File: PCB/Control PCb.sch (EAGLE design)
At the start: 7 parts

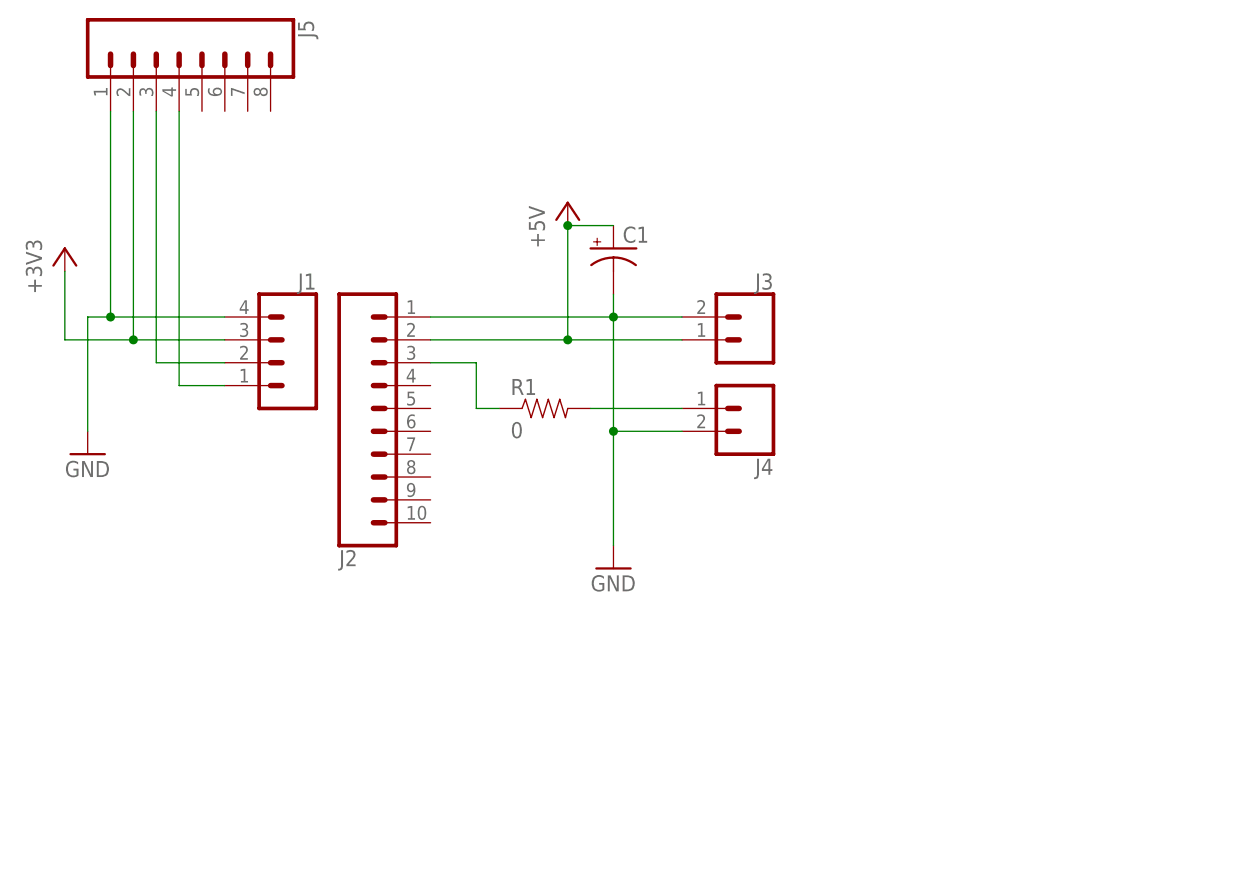
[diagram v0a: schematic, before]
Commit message: PCB files etc
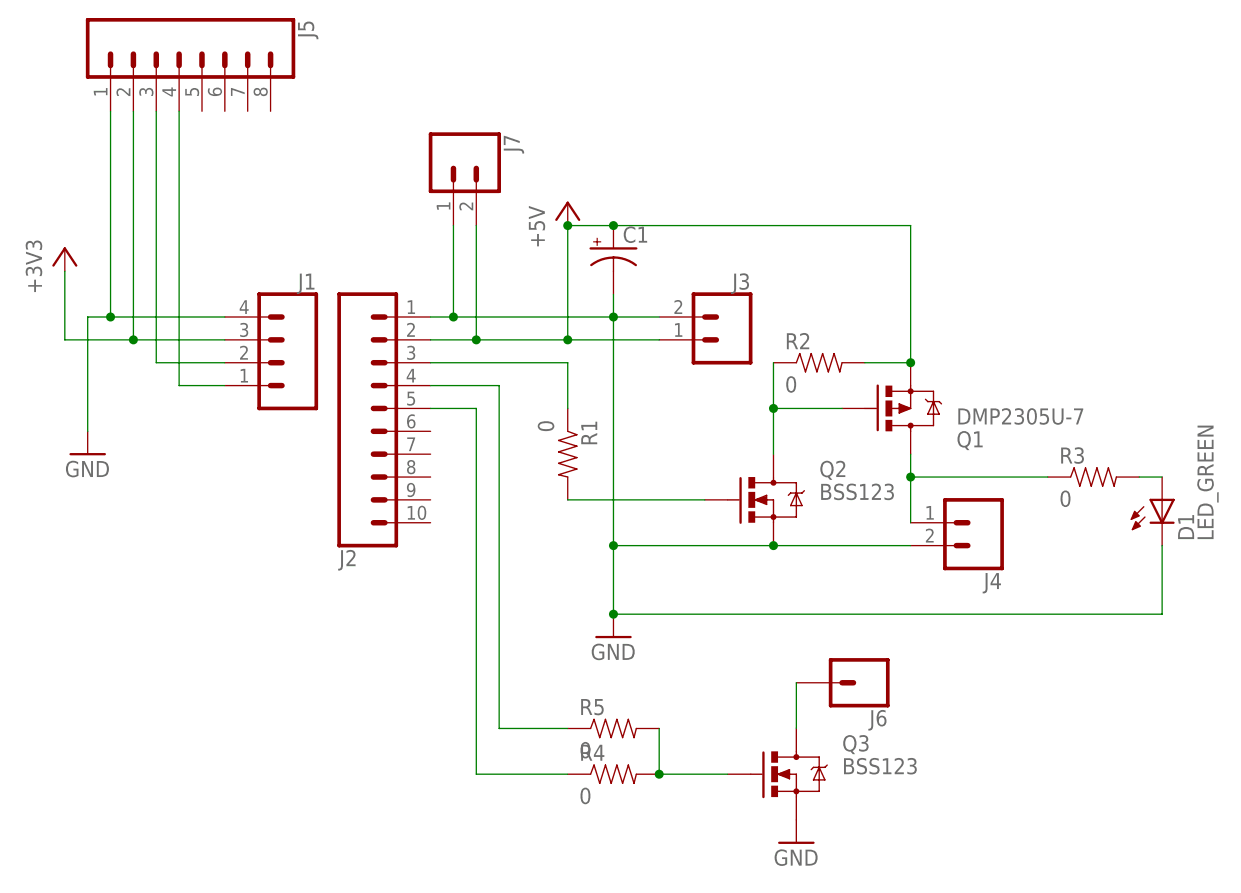
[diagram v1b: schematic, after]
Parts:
- added D1: LED_GREEN, RJC-2:LED_GREEN
- added J6: (no value), SparkFun-Connectors:CONN_01OFFSET
- added J7: (no value), SparkFun-Connectors:CONN_02LOCK_LONGPADS
- added Q1: DMP2305U-7, RJC-2:MOS-P_DMP2305U-7
- added Q2, Q3: BSS123, RJC-2:MOS-N_BSS123
- added R2, R3, R4, R5: 0, RJC-2:RES_0_0805
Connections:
- new net N$10: J2.4, R5.1
- new net N$11: J6.1, Q3.D
- new net N$5: Q1.G, Q2.D, R2.1
- new net N$6: J4.1, Q1.D, R3.1
- new net N$7: D1.A, R3.2
- new net N$8: Q3.G, R4.2, R5.2
- new net N$9: J2.5, R4.1
- net +5V: now also J7.2, Q1.S, R2.2
- net GND: now also D1.C, J7.1, Q2.S, Q3.S
- net N$2: now also Q2.G; no longer J4.1
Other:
- moved on the sheet: J3, J4, R1
